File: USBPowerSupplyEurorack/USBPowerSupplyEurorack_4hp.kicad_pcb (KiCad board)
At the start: 2 copper layers, 19.9 x 110 mm, 36 parts, among them J1 1734366-1, J2 95278-501A10LF, Q1 Q_PMOS_GSD

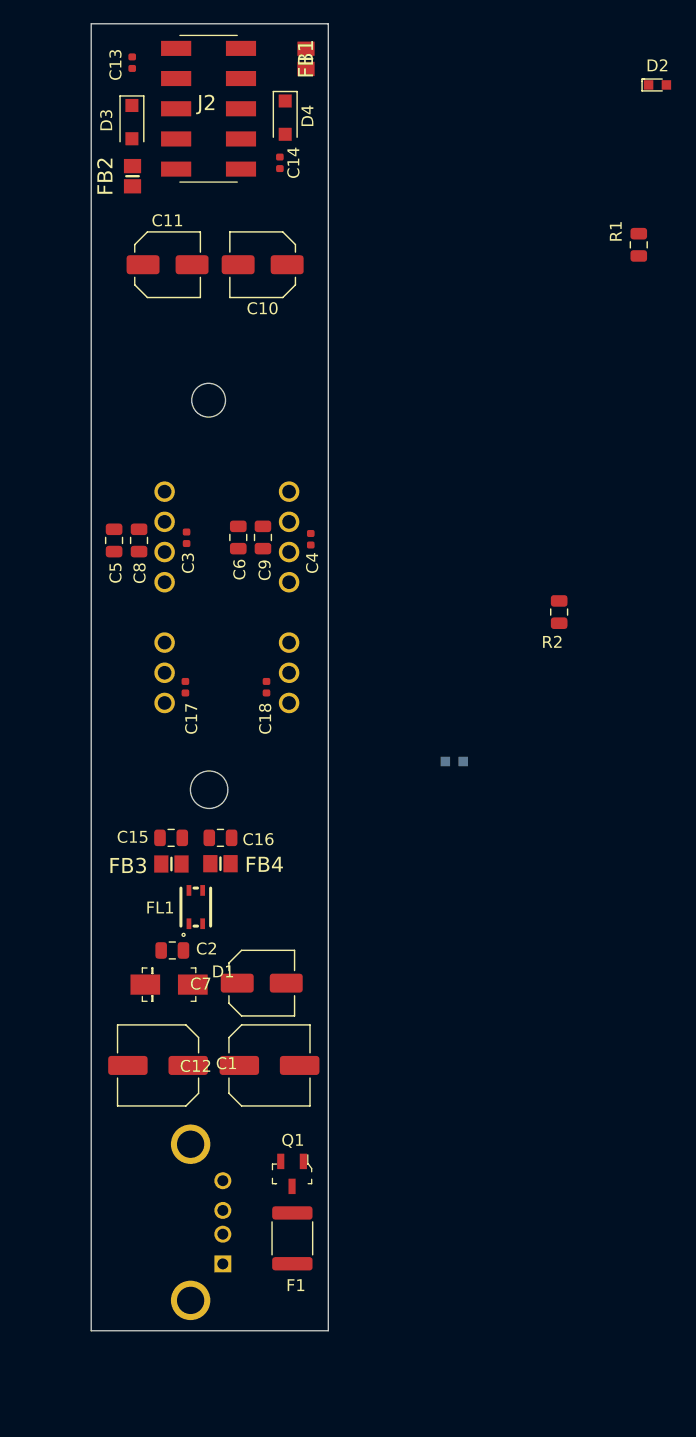
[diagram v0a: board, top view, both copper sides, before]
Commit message: still testing routing
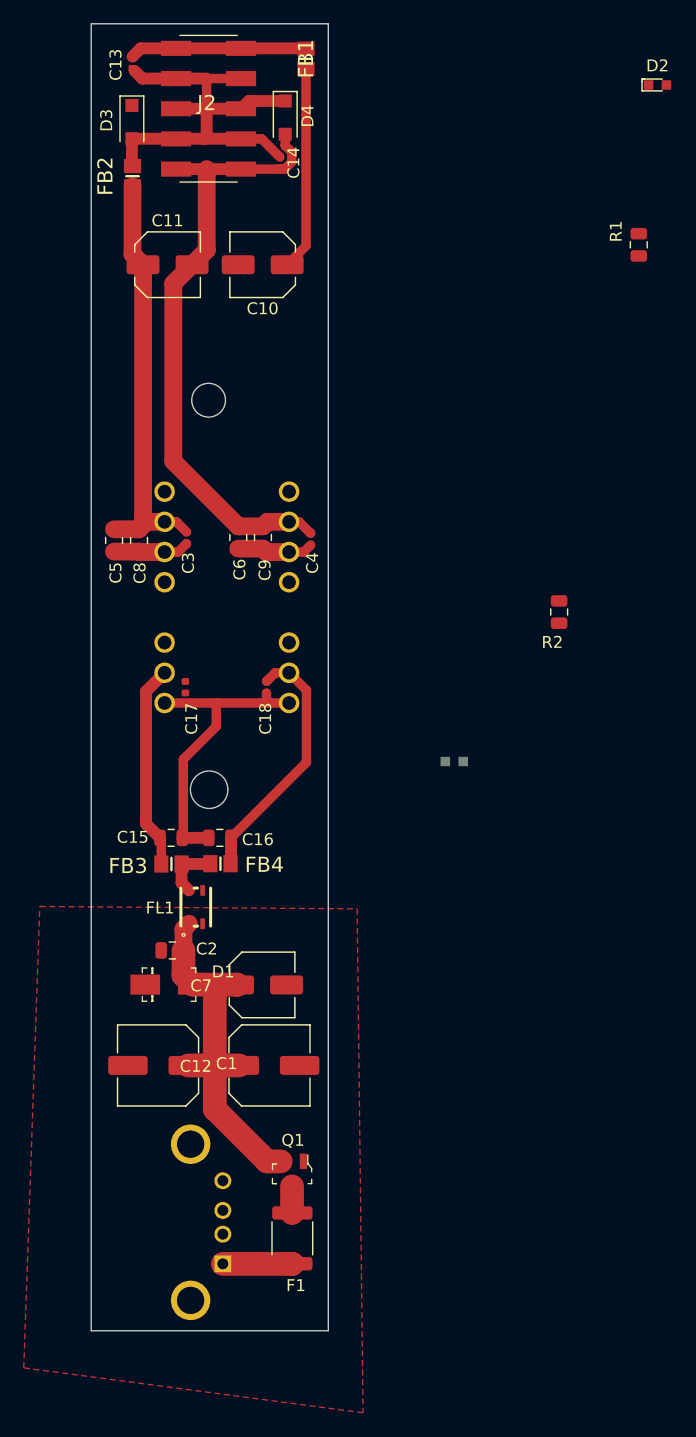
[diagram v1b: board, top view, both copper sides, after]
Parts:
- moved C7 0.15 mm to (143.9, 129.0)
- moved C16 0.05 mm to (140.4, 116.6)
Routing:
- net -12V: track 0.00 -> 52.7 mm
- net 0V: track 0.00 -> 41.9 mm
- net Net-(C13-Pad2): track 0.00 -> 39.2 mm
- net Net-(C1-Pad1): track 0.00 -> 31.6 mm
- net -Vin1: track 0.00 -> 26.1 mm
- net +12V: track 0.00 -> 23.5 mm
- net +Vin2: track 0.00 -> 21.5 mm
- net +Vin1: track 0.00 -> 17.3 mm
- net Net-(C13-Pad1): track 0.00 -> 14.9 mm
- net Net-(F1-Pad1): track 0.00 -> 5.86 mm
- net Net-(FB3-Pad2): track 0.00 -> 4.92 mm
- net +5V: track 0.00 -> 2.25 mm
- added copper zone on F.Cu, net GND
